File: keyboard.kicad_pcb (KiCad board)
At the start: 2 copper layers, 333.4 x 114.3 mm, 192 parts, among them SW1 SW_Push, U1 ATmega32U4-AU, Y1 16MHz

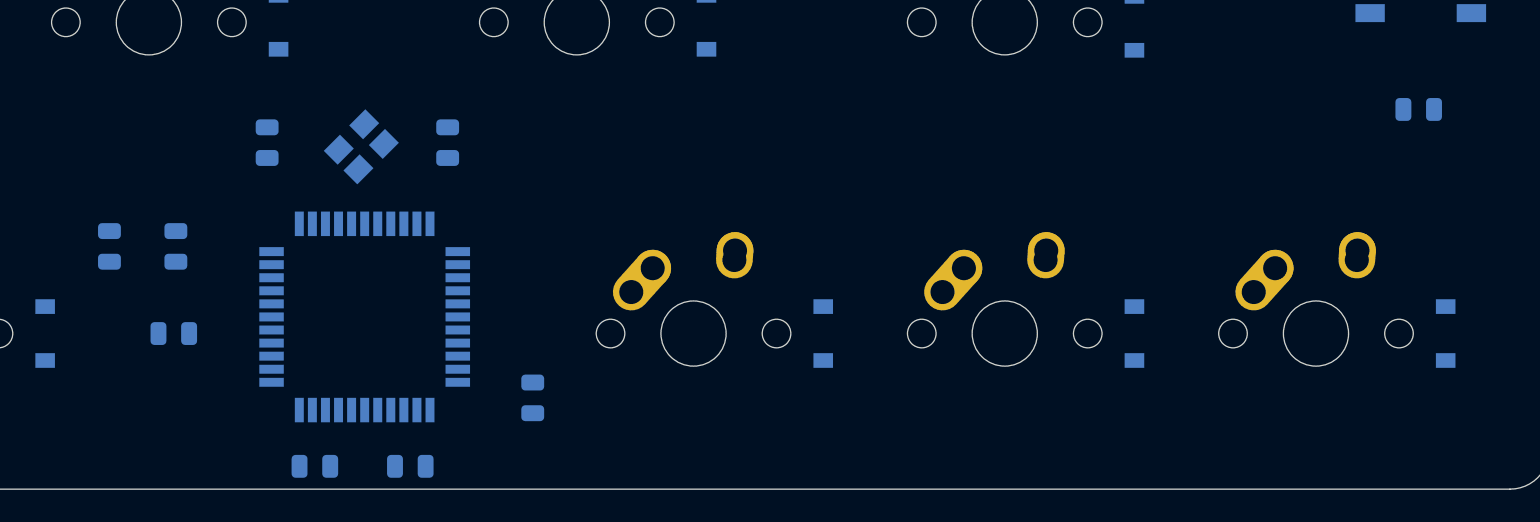
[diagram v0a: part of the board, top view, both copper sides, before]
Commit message: Placement and prepare for routing
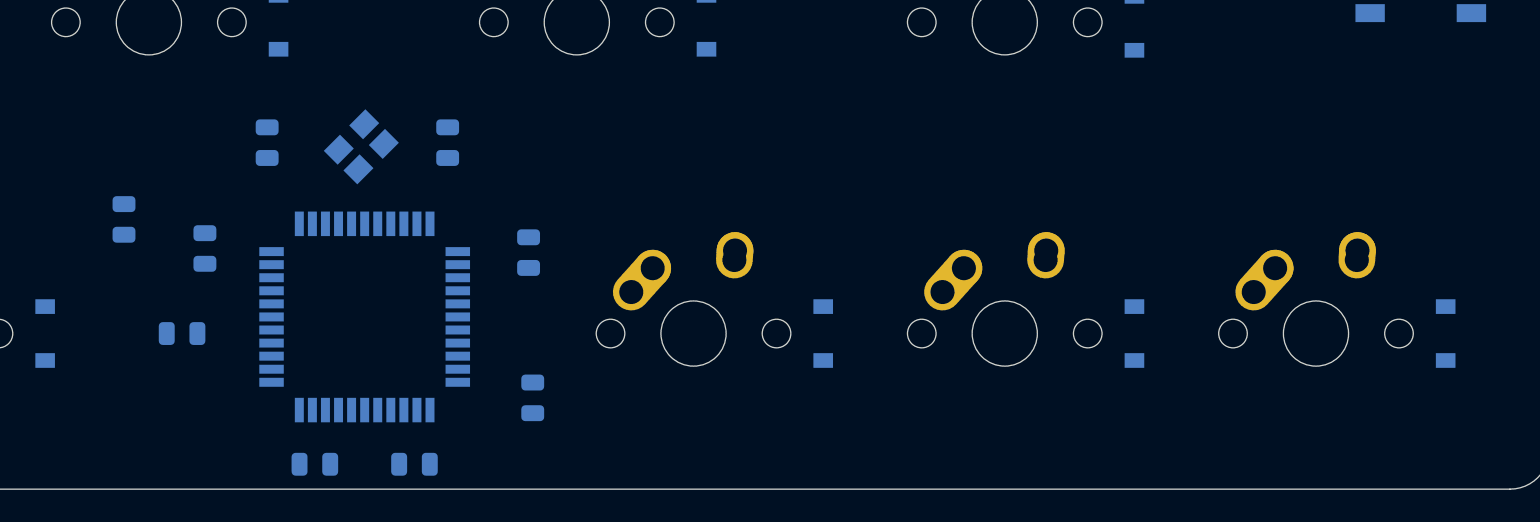
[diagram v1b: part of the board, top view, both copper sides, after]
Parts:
- moved R3 79.5 mm to (236.6, 88.3), turned to 270 degrees
- moved C1 25.7 mm to (261.4, 90.3)
- moved C5 6.10 mm to (254.4, 103.3)
- moved C6 5.84 mm to (248.3, 103.3), turned to 0 degrees
- moved C2 1.78 mm to (241.6, 90.0)
- moved C7 0.51 mm to (240.2, 95.2)
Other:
- net class Default: trace_width 0.25 -> 0.254
- net class Power added: clearance 0.2, trace_width 0.381, via_dia 0.8, via_drill 0.4
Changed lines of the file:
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@@
   )
   (setup
-    (last_trace_width 0.25)
+    (last_trace_width 0.254)
     (trace_clearance 0.2)
     (zone_clearance 0.508)
@@
   (net_class Default "This is the default net class."
     (clearance 0.2)
-    (trace_width 0.25)
+    (trace_width 0.254)
     (via_dia 0.8)
     (via_drill 0.4)
     (uvia_dia 0.3)
     (uvia_drill 0.1)
-    (add_net +5V)
     (add_net COL0)
     (add_net COL1)
@@
     (add_net D+)
     (add_net D-)
-    (add_net GND)
     (add_net "Net-(C3-Pad1)")
     (add_net "Net-(C4-Pad1)")
@@
     (add_net ROW4)
     (add_net ROW5)
+  )
+  (net_class Power ""
+    (clearance 0.2)
+    (trace_width 0.381)
+    (via_dia 0.8)
+    (via_drill 0.4)
+    (uvia_dia 0.3)
+    (uvia_drill 0.1)
+    (add_net +5V)
+    (add_net GND)
     (add_net VCC)
   )
@@
   )
   (module Resistor_SMD:R_0805_2012Metric (layer B.Cu)
-    (at 315.849 81.534)
+    (at 236.601 88.265 270)
     (descr "Resistor SMD 0805 (2012 Metric), square (rectangular) end terminal, IPC_7351 nominal, (Body size source: https://docs.google.com/spreadsheets/d/1BsfQQcO9C6DZCsRaXUlFlo91Tg2WpOkGARC1WS5S8t0/edit?usp=sharing), generated with kicad-footprint-generator")
     (tags resistor)
     (attr smd)
-    (fp_text reference R3 (at 0 1.65) (layer B.SilkS)
+    (fp_text reference R3 (at 0 1.65 90) (layer B.SilkS)
       (effects (font (size 1 1) (thickness 0.15)) (justify mirror))
     )
-    (fp_text value 10k (at 0 -1.65) (layer B.Fab)
+    (fp_text value 10k (at 0 -1.65 90) (layer B.Fab)
       (effects (font (size 1 1) (thickness 0.15)) (justify mirror))
     )
-    (fp_text user %R (at 0 0) (layer B.Fab)
+    (fp_text user %R (at 0 0 90) (layer B.Fab)
       (effects (font (size 0.5 0.5) (thickness 0.08)) (justify mirror))
     )
@@
     (fp_line (start -1 0.6) (end 1 0.6) (layer B.Fab) (width 0.1))
     (fp_line (start -1 -0.6) (end -1 0.6) (layer B.Fab) (width 0.1))
-    (pad 2 smd roundrect (at 0.9375 0) (size 0.975 1.4) (layers B.Cu B.Paste B.Mask) (roundrect_rratio 0.25)
+    (pad 2 smd roundrect (at 0.9375 0 270) (size 0.975 1.4) (layers B.Cu B.Paste B.Mask) (roundrect_rratio 0.25)
       (net 2 +5V))
-    (pad 1 smd roundrect (at -0.9375 0) (size 0.975 1.4) (layers B.Cu B.Paste B.Mask) (roundrect_rratio 0.25)
+    (pad 1 smd roundrect (at -0.9375 0 270) (size 0.975 1.4) (layers B.Cu B.Paste B.Mask) (roundrect_rratio 0.25)
       (net 122 "Net-(R3-Pad1)"))
     (model ${KISYS3DMOD}/Resistor_SMD.3dshapes/R_0805_2012Metric.wrl
@@
   )
   (module Capacitor_SMD:C_0805_2012Metric (layer B.Cu)
-    (at 239.649 95.25 180)
+    (at 240.157 95.25 180)
     (descr "Capacitor SMD 0805 (2012 Metric), square (rectangular) end terminal, IPC_7351 nominal, (Body size source: https://docs.google.com/spreadsheets/d/1BsfQQcO9C6DZCsRaXUlFlo91Tg2WpOkGARC1WS5S8t0/edit?usp=sharing), generated with kicad-footprint-generator")
     (tags capacitor)
@@
   )
   (module Capacitor_SMD:C_0805_2012Metric (layer B.Cu)
-    (at 254.127 103.378 180)
+    (at 248.285 103.251)
     (descr "Capacitor SMD 0805 (2012 Metric), square (rectangular) end terminal, IPC_7351 nominal, (Body size source: https://docs.google.com/spreadsheets/d/1BsfQQcO9C6DZCsRaXUlFlo91Tg2WpOkGARC1WS5S8t0/edit?usp=sharing), generated with kicad-footprint-generator")
     (tags capacitor)
@@
     (fp_line (start -1 0.6) (end 1 0.6) (layer B.Fab) (width 0.1))
     (fp_line (start -1 -0.6) (end -1 0.6) (layer B.Fab) (width 0.1))
-    (pad 2 smd roundrect (at 0.9375 0 180) (size 0.975 1.4) (layers B.Cu B.Paste B.Mask) (roundrect_rratio 0.25)
+    (pad 2 smd roundrect (at 0.9375 0) (size 0.975 1.4) (layers B.Cu B.Paste B.Mask) (roundrect_rratio 0.25)
       (net 1 GND))
-    (pad 1 smd roundrect (at -0.9375 0 180) (size 0.975 1.4) (layers B.Cu B.Paste B.Mask) (roundrect_rratio 0.25)
+    (pad 1 smd roundrect (at -0.9375 0) (size 0.975 1.4) (layers B.Cu B.Paste B.Mask) (roundrect_rratio 0.25)
       (net 2 +5V))
     (model ${KISYS3DMOD}/Capacitor_SMD.3dshapes/C_0805_2012Metric.wrl
@@
   )
   (module Capacitor_SMD:C_0805_2012Metric (layer B.Cu)
-    (at 248.285 103.378 180)
+    (at 254.381 103.251 180)
     (descr "Capacitor SMD 0805 (2012 Metric), square (rectangular) end terminal, IPC_7351 nominal, (Body size source: https://docs.google.com/spreadsheets/d/1BsfQQcO9C6DZCsRaXUlFlo91Tg2WpOkGARC1WS5S8t0/edit?usp=sharing), generated with kicad-footprint-generator")
     (tags capacitor)
@@
   )
   (module Capacitor_SMD:C_0805_2012Metric (layer B.Cu)
-    (at 239.776 89.916 90)
+    (at 241.554 90.043 90)
     (descr "Capacitor SMD 0805 (2012 Metric), square (rectangular) end terminal, IPC_7351 nominal, (Body size source: https://docs.google.com/spreadsheets/d/1BsfQQcO9C6DZCsRaXUlFlo91Tg2WpOkGARC1WS5S8t0/edit?usp=sharing), generated with kicad-footprint-generator")
     (tags capacitor)
@@
   )
   (module Capacitor_SMD:C_0805_2012Metric (layer B.Cu)
-    (at 235.712 89.916 90)
+    (at 261.366 90.297 90)
     (descr "Capacitor SMD 0805 (2012 Metric), square (rectangular) end terminal, IPC_7351 nominal, (Body size source: https://docs.google.com/spreadsheets/d/1BsfQQcO9C6DZCsRaXUlFlo91Tg2WpOkGARC1WS5S8t0/edit?usp=sharing), generated with kicad-footprint-generator")
     (tags capacitor)
